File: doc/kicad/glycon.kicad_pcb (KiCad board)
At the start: 2 copper layers, 200 x 100 mm, 39 parts, among them IC1 SIO0-DIP-40, IC2 CTC-DIP-28, J1 Arduino/system bus header, J2 PMOD USBUART conn, J3 Int order hdr, J4 Conn_02x21_Odd_Even, SW1 SW_Push_Open, U0 Z80CPU, U1 628128_DIP32_SSOP32, U10 74HC244, U11 PIO-DIP-40, U12 74LS21, U2 SST39SF010, U3 74HC32, U4 74HC04, U6 74LS139, U7 SIO0-DIP-40, U9 74HC244, X1 ACO-6.00MHz

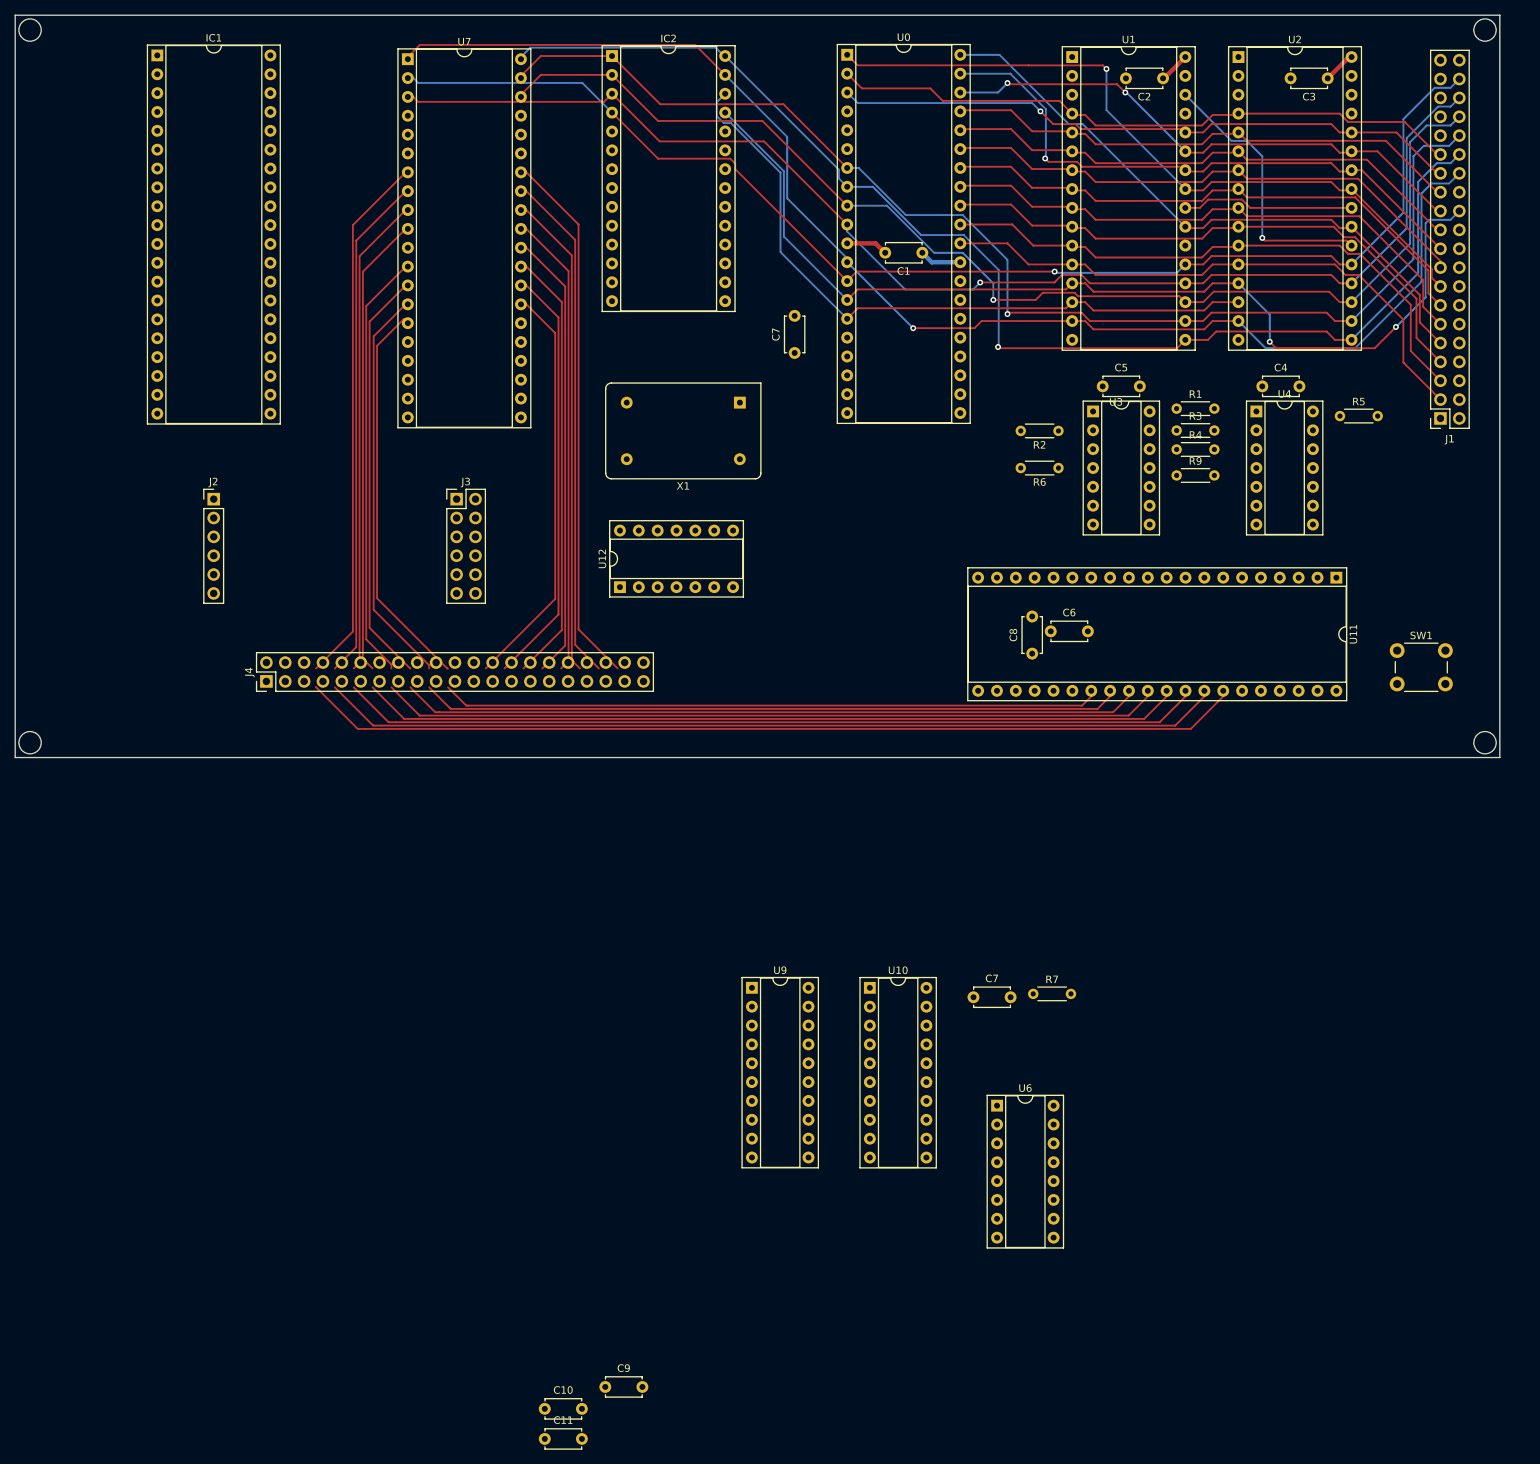
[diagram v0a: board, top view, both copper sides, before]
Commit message: more pcb work
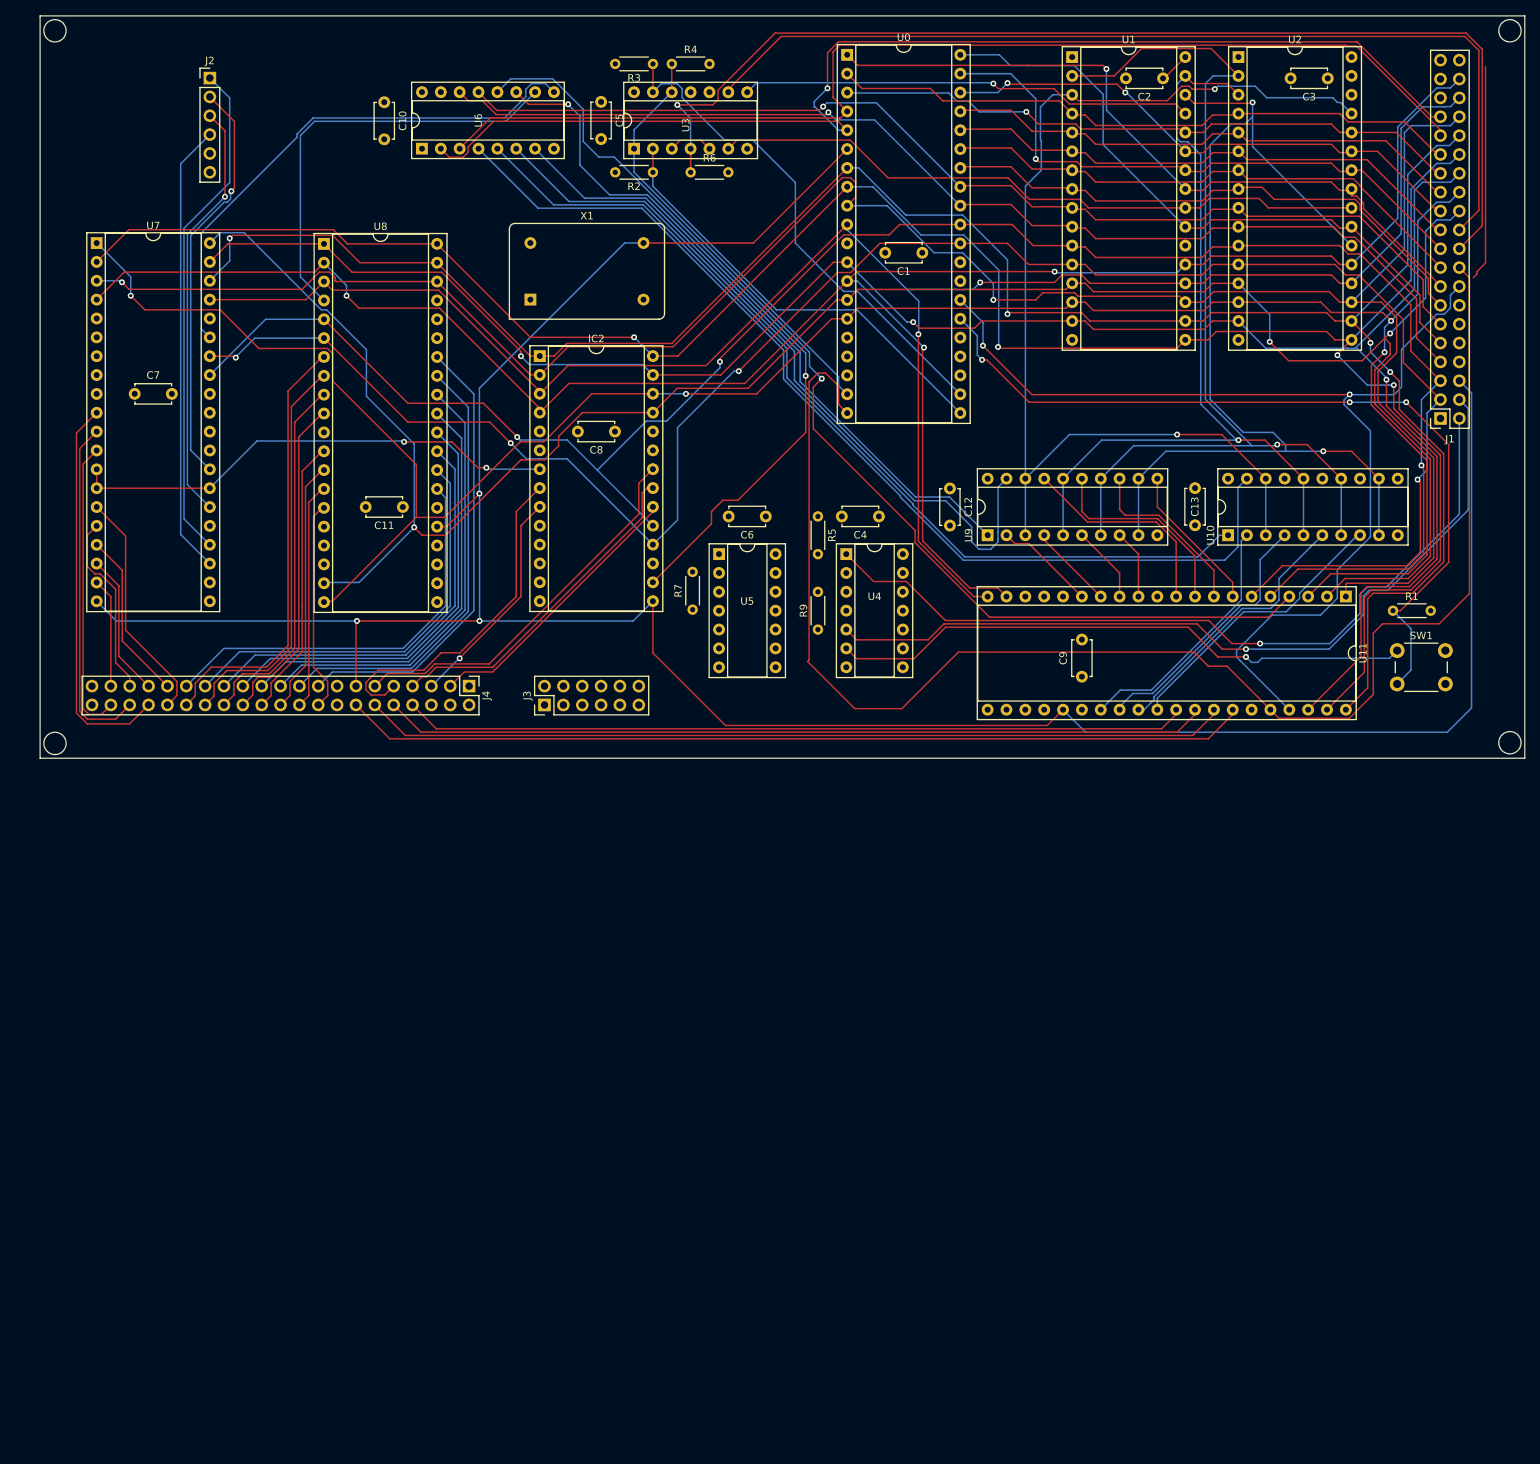
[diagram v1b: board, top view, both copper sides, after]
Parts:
- removed the C7 at (125.0, 65.5)
- removed the C7 at (149.1, 152.3)
- removed IC1: SIO0-DIP-40, Package_DIP:DIP-40_W15.24mm_Socket
- removed U12: 74LS21, Package_DIP:DIP-14_W7.62mm_Socket
- added C12: 100nF, Capacitor_THT:C_Disc_D4.7mm_W2.5mm_P5.00mm, F.Cu at (145.9, 83.8)
- added C13: 100nF, Capacitor_THT:C_Disc_D4.7mm_W2.5mm_P5.00mm, F.Cu at (178.9, 83.7)
- added C7: 100nF, Capacitor_THT:C_Disc_D4.7mm_W2.5mm_P5.00mm, F.Cu at (36.1, 71.0)
- added U5: 74LS21, Package_DIP:DIP-14_W7.62mm_Socket, F.Cu at (114.8, 92.6)
- added U8: PIO-DIP-40, Package_DIP:DIP-40_W15.24mm_Socket, F.Cu at (61.6, 50.8)
- moved C10 177.3 mm to (69.7, 31.7), turned to -90 degrees
- moved U6 150.4 mm to (74.8, 38.0), turned to 90 degrees
- moved C11 127.0 mm to (72.2, 86.2), turned to 180 degrees
- moved C9 115.2 mm to (163.7, 109.1), turned to 90 degrees
- moved R3 86.1 mm to (105.9, 26.6), turned to 180 degrees
- moved R4 85.6 mm to (108.5, 26.6)
- moved U10 77.8 mm to (183.4, 90.0), turned to 90 degrees
- moved C5 77.7 mm to (98.9, 31.7), turned to -90 degrees
- moved R5 71.6 mm to (128.1, 87.5), turned to -90 degrees
- moved U3 71.2 mm to (103.4, 38.0), turned to 90 degrees
- moved R7 69.2 mm to (111.3, 100.1), turned to 90 degrees
- moved U9 68.7 mm to (151.0, 90.0), turned to 90 degrees
- moved R2 64.8 mm to (105.9, 41.2)
- moved C8 63.7 mm to (100.8, 76.1), turned to 180 degrees
- moved R6 63.6 mm to (111.0, 41.2), turned to 0 degrees
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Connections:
- net Net-(U6B-O3) renamed /~{IO_EN1}
- IC2 pad 6: /CLK -> /~{IORD}
- J1 pad 1: VDD -> +5V
- J1 pad 6: unconnected-(J1-Pin_6) -> /CLK
- J2 pad 6: VCC -> /VIN
- J4 pad 1: VDD -> +5V
- J4 pad 15: VDD -> +5V
- J4 pad 17: /PA7 -> /PB7
- J4 pad 18: /PB0 -> /PA0
- J4 pad 19: /PA6 -> /PB6
- J4 pad 20: /PB1 -> /PA1
- J4 pad 21: /PA5 -> /PB5
- J4 pad 22: /PB2 -> /PA2
- J4 pad 23: /PA4 -> /PB4
- J4 pad 24: /PB3 -> /PA3
- J4 pad 25: /PA3 -> /PB3
- J4 pad 26: /PB4 -> /PA4
- J4 pad 27: /PA2 -> /PB2
- J4 pad 28: /PB5 -> /PA5
- J4 pad 29: /PA1 -> /PB1
- J4 pad 30: /PB6 -> /PA6
- J4 pad 31: /PA0 -> /PB0
- J4 pad 32: /PB7 -> /PA7
- J4 pad 36: /SERCLK -> /~{W}/~{RDYA}
- J4 pad 4: /RESET -> /VIN
- J4 pad 40: /~{W}/~{RDYA} -> /RXDA
- J4 pad 41: VDD -> +5V
- J4 pad 6: unconnected-(J4-Pin_6) -> /RESET
- R2 pad 1: /CLK -> /~{RD}
- U0 pad 21: /CLK -> /~{RD}
- U1 pad 30: /A18 -> /A17
- U11 pad 35: /CLK -> /~{IORD}
- U2 pad 22: unconnected-(U2-~{CE}) -> /A17
- U3 pad 2: /CLK -> /~{RD}
- U7 pad 12: unconnected-(U7-RXDA) -> /RXDA
- U7 pad 32: /CLK -> /~{IORD}
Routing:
- net /CLK: track 65.5 -> 357.3 mm, vias 0 -> 3
- net /D1: track 93.2 -> 305.0 mm, vias 0 -> 4
- net /~{IORQ}: track 0.00 -> 202.0 mm
- net /D0: track 135.7 -> 297.0 mm, vias 2 -> 3
- net /PGA1: track 0.00 -> 159.3 mm, vias 0 -> 1
- net /RAM/ROM OE: track 0.00 -> 152.1 mm, vias 0 -> 1
- net /PGA0: track 0.00 -> 150.8 mm
- net /A14: track 0.00 -> 149.1 mm, vias 0 -> 2
- net Net-(U11-~{CE}): track 0.00 -> 148.8 mm, vias 0 -> 1
- net /~{RESET}: track 0.00 -> 141.2 mm, vias 0 -> 3
- net /A17: track 0.00 -> 140.2 mm, vias 0 -> 2
- net Net-(U10-2OE): track 0.00 -> 138.1 mm
- net /D3: track 169.2 -> 304.1 mm, vias 1 -> 4
- net /A16: track 0.00 -> 133.1 mm, vias 0 -> 1
- net /D5: track 161.5 -> 293.7 mm, vias 1 -> 2
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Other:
- outline, holes or cut-outs redrawn
